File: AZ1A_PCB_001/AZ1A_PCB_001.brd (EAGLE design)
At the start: 160 x 120 mm, 35 parts

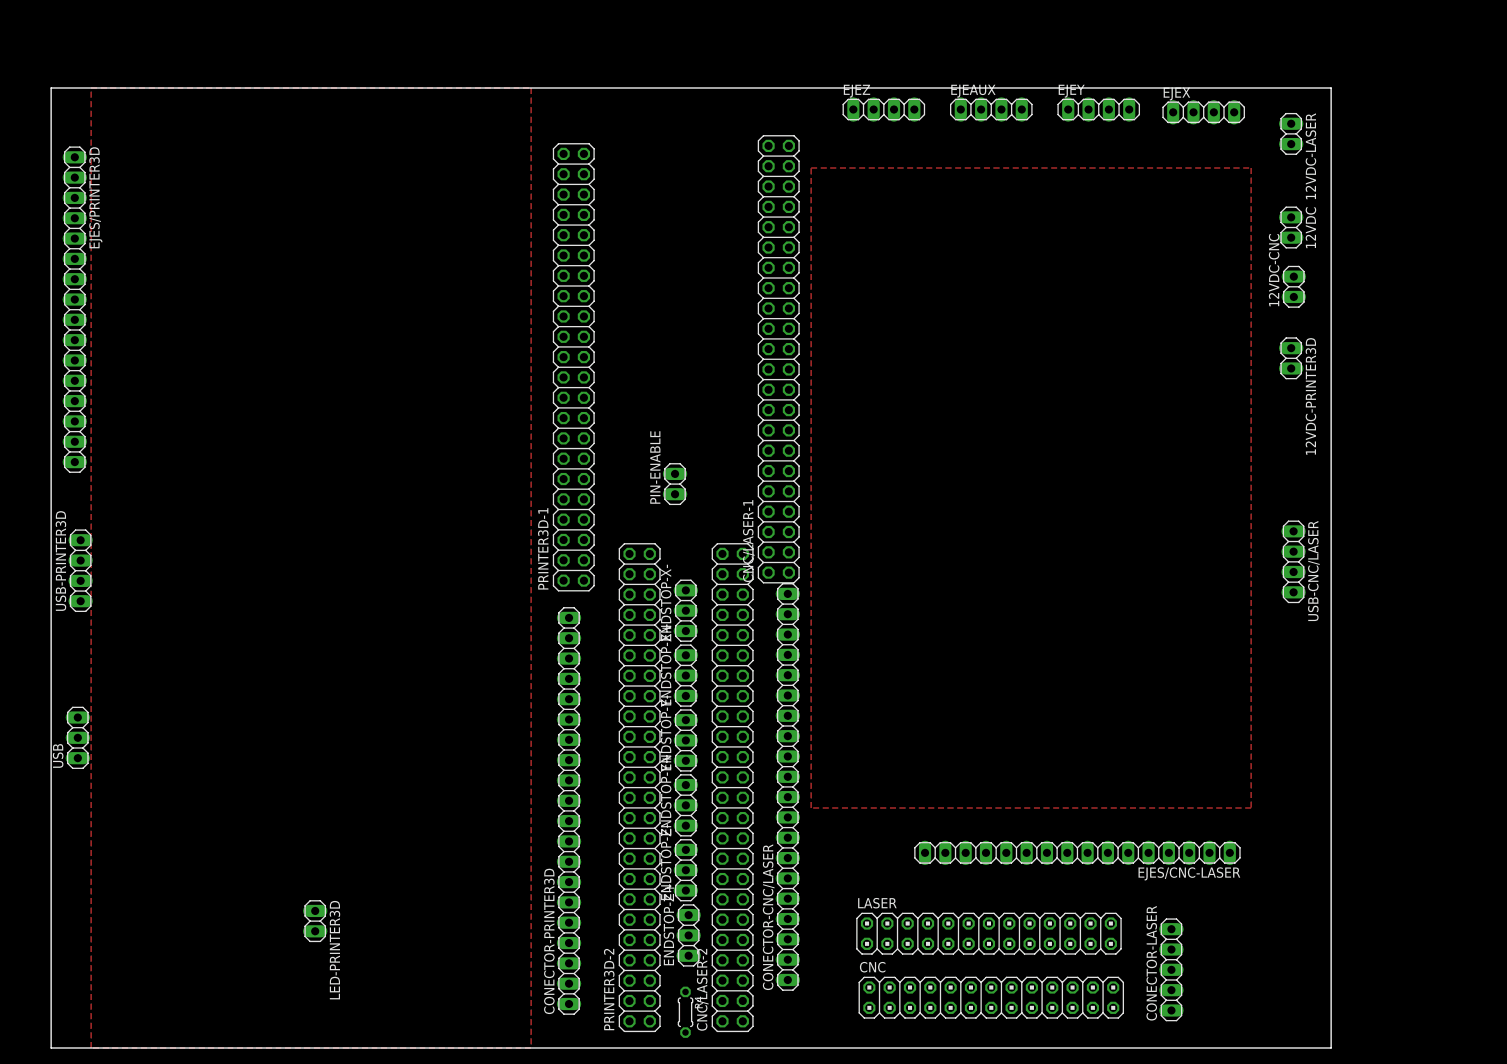
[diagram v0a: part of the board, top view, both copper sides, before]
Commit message: Actualización de PCB
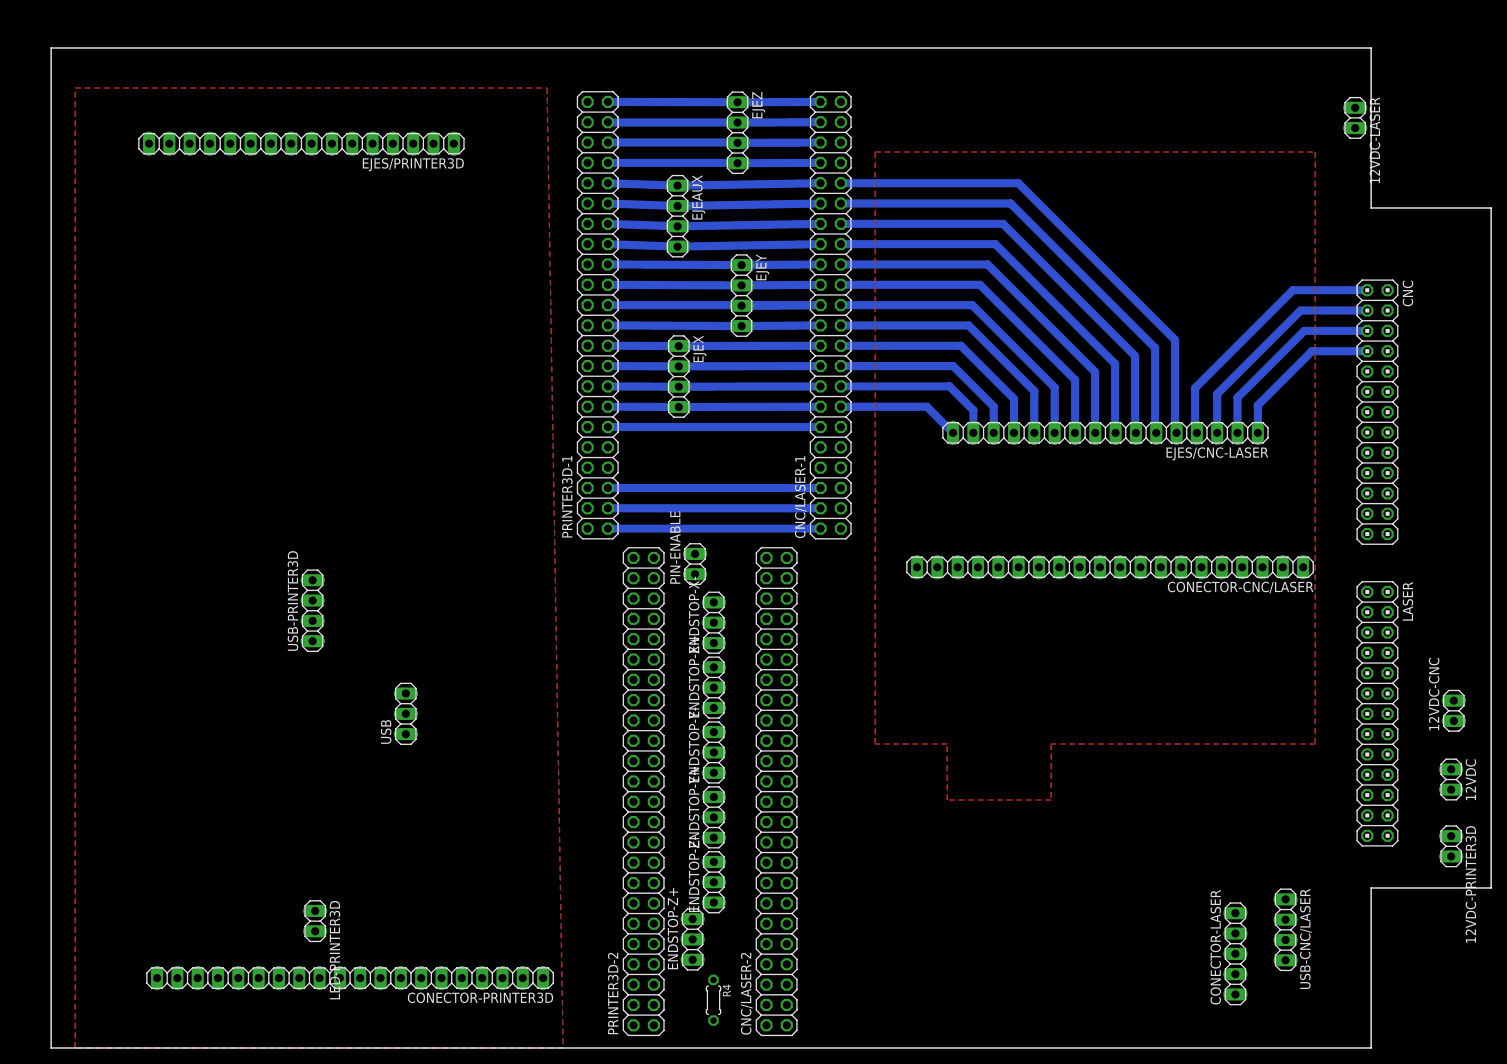
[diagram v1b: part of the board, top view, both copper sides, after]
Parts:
- moved CNC 87.7 mm to (165.8, 79.5), turned to 270 degrees
- moved EJEX 73.5 mm to (78.5, 83.9), turned to 270 degrees
- moved 12VDC 71.8 mm to (175.0, 33.6)
- moved 12VDC-PRINTER3D 64.2 mm to (175.0, 25.2)
- moved 12VDC-CNC 56.6 mm to (175.3, 42.1)
- moved LASER 55.8 mm to (165.8, 41.8), turned to 270 degrees
- moved EJES/CNC-LASER 52.6 mm to (131.8, 76.9)
- moved EJEY 50.3 mm to (86.3, 94.0), turned to 270 degrees
- moved CONECTOR-CNC/LASER 48.7 mm to (132.4, 60.1), turned to 180 degrees
- moved USB-CNC/LASER 46.0 mm to (154.3, 14.8)
- moved EJEAUX 41.4 mm to (78.3, 104.0), turned to 270 degrees
- moved USB 41.1 mm to (44.3, 41.8)
- moved EJES/PRINTER3D 35.1 mm to (31.3, 113.0), turned to 180 degrees
- moved CONECTOR-PRINTER3D 34.4 mm to (37.4, 8.74), turned to 180 degrees
- moved USB-PRINTER3D 29.4 mm to (32.7, 54.7)
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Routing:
- net N$47: track 0.00 -> 61.6 mm
- net N$48: track 0.00 -> 57.4 mm
- net N$49: track 0.00 -> 53.3 mm
- net N$50: track 0.00 -> 49.1 mm
- net N$51: track 0.00 -> 45.0 mm
- net N$52: track 0.00 -> 40.8 mm
- net N$53: track 0.00 -> 36.7 mm
- net N$6: track 0.00 -> 36.5 mm
- net N$54: track 0.00 -> 32.8 mm
- net N$21: track 0.00 -> 32.3 mm
- net N$57: track 0.00 -> 28.6 mm
- net N$24: track 0.00 -> 27.9 mm
- net N$14: track 0.00 -> 27.0 mm
- net N$13: track 0.00 -> 26.6 mm
- net N$15: track 0.00 -> 26.6 mm
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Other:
- board size 160 x 120 mm -> 180 x 125 mm
